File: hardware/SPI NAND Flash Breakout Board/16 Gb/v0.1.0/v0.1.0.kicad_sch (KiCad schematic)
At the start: 5 parts, among them J1 Conn_01x09_Pin, U1 AS5F18G04SND-10LIN, U2 TXB0108PW, U3 AS5F18G04SND-10LIN, U4 AP2127K-1.8

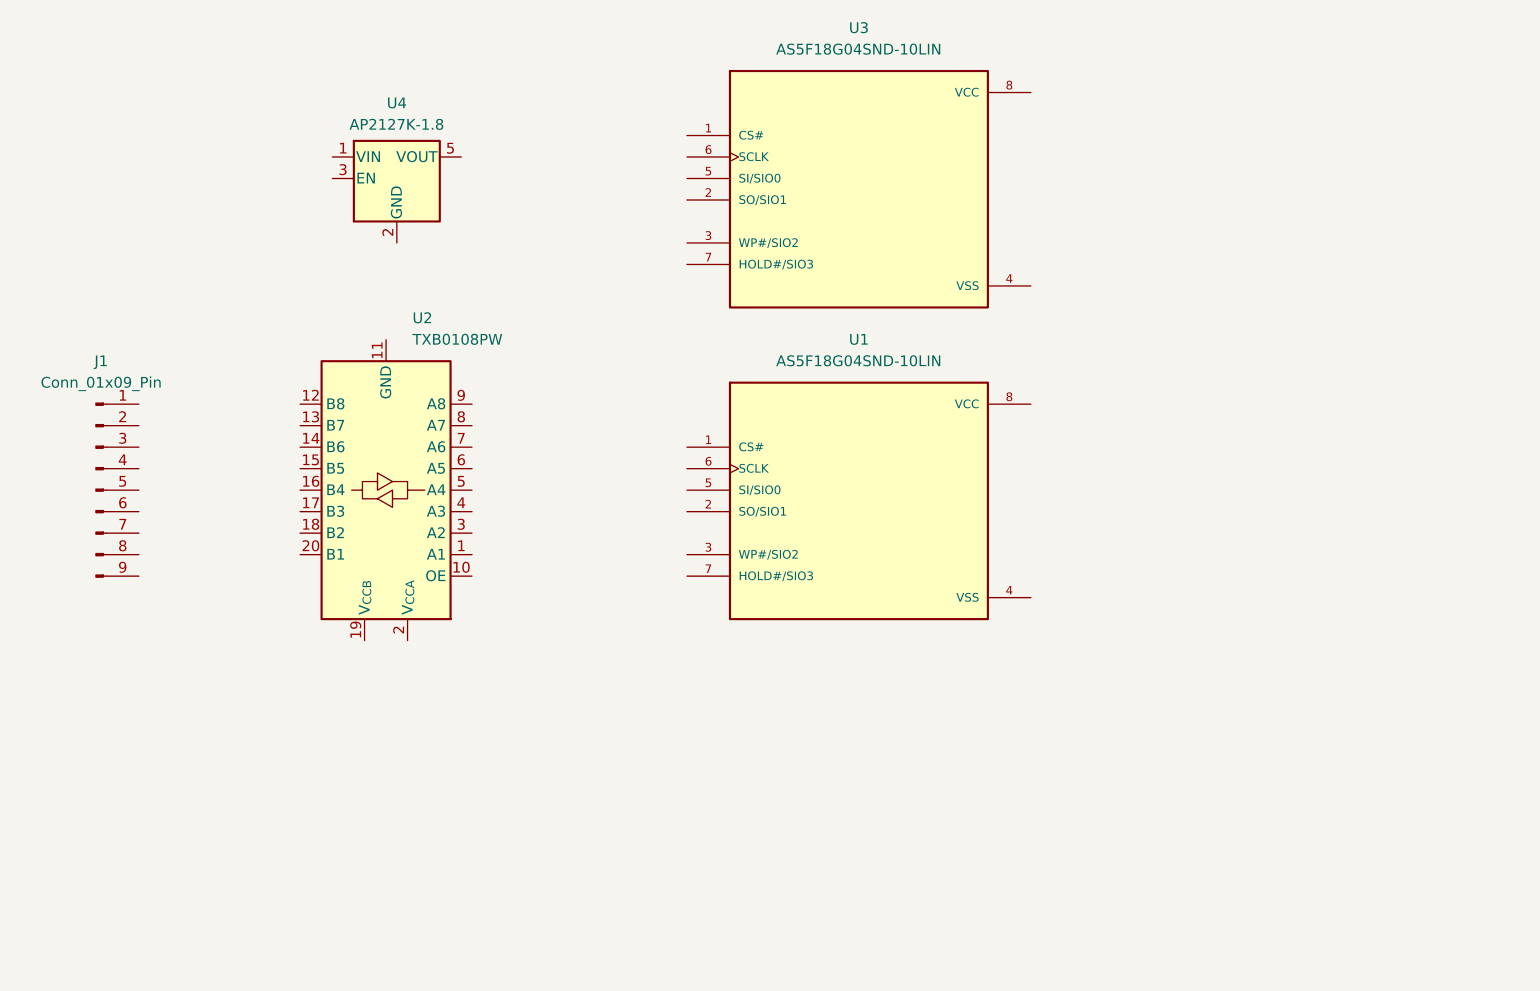
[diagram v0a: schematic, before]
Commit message: 16 Gb Design
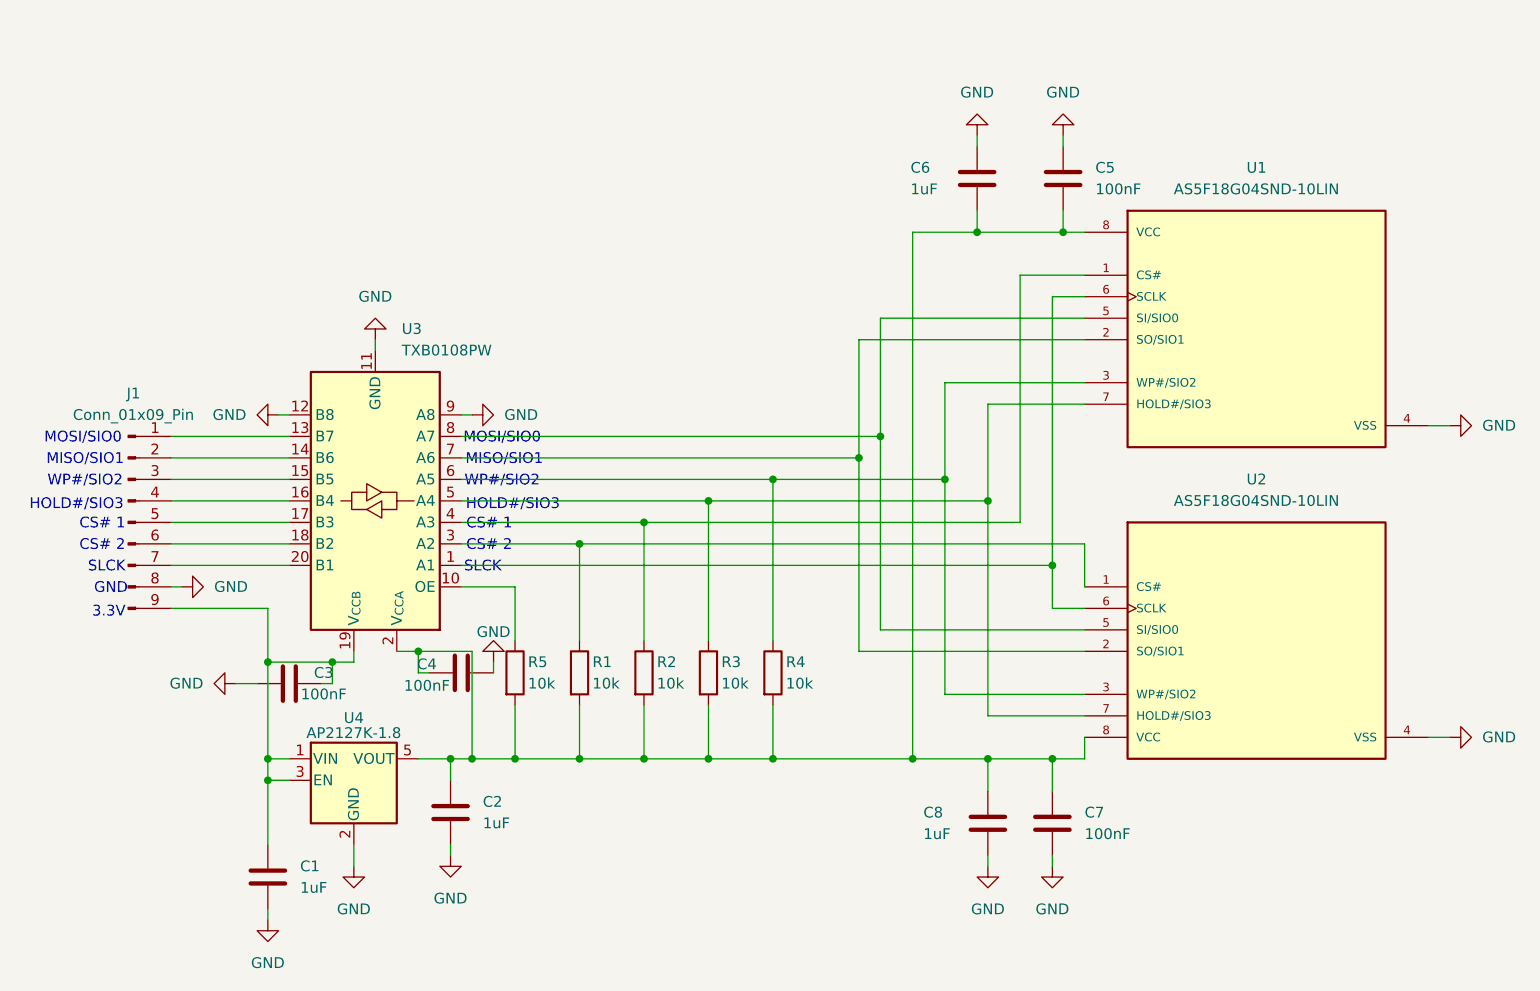
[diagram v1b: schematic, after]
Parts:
- added C1, C2, C6, C8: 1uF, Capacitor_SMD:C_0805_2012Metric, symbol Device:C
- added C3, C4, C5, C7: 100nF, Capacitor_SMD:C_0805_2012Metric, symbol Device:C
- added R1, R2, R3, R4, R5: 10k, Resistor_SMD:R_0805_2012Metric, symbol Device:R
- J1: footprint (none) -> Connector_PinSocket_2.54mm:PinSocket_1x09_P2.54mm_Vertical
- U1: renamed from U3; footprint AS5F18G04SND-10LIN:SON127P600X800X80-8N -> Breakout:SON127P600X800X80-8N
- U2: renamed from U1; footprint AS5F18G04SND-10LIN:SON127P600X800X80-8N -> Breakout:SON127P600X800X80-8N
- renumbered U2 to U3
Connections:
- net at U2.1 (CS#): now also U3.3 (A2), R1.1
- net at U2.2 (SO/SIO1): now also U1.2 (SO/SIO1), U3.7 (A6)
- net at U2.3 (WP#/SIO2): now also U1.3 (WP#/SIO2), U3.6 (A5), R4.1
- net GND: now reaches U2.4 (VSS)
- net GND: now also J1.8 (Pin_8), U1.4 (VSS), U3.11 (GND), U3.12 (B8), U3.9 (A8), U4.2 (GND), C1.2, C2.2, C3.1, C4.1, C5.1, C6.1, C7.2, C8.2
- net at U2.5 (SI/SIO0): now also U1.5 (SI/SIO0), U3.8 (A7)
- net at U2.6 (SCLK): now also U1.6 (SCLK), U3.1 (A1)
- net at U2.7 (HOLD#/SIO3): now also U1.7 (HOLD#/SIO3), U3.5 (A4), R3.1
- net at U2.8 (VCC): now also U1.8 (VCC), U3.2 (V_{CCA}), U4.5 (VOUT), C2.1, C4.2, C5.2, C6.2, C7.1, C8.1, R1.2, R2.2, R3.2, R4.2, R5.2
- net at J1.1 (Pin_1): now also U3.13 (B7)
- net at J1.2 (Pin_2): now also U3.14 (B6)
- net at J1.3 (Pin_3): now also U3.15 (B5)
- net at J1.4 (Pin_4): now also U3.16 (B4)
- net at J1.5 (Pin_5): now also U3.17 (B3)
- net at J1.6 (Pin_6): now also U3.18 (B2)
- net at J1.7 (Pin_7): now also U3.20 (B1)
- net at J1.9 (Pin_9): now also U3.19 (V_{CCB}), U4.1 (VIN), U4.3 (EN), C1.1, C3.2
- net at U3.10 (OE): now also R5.1
- net at U3.4 (A3): now also U1.1 (CS#), R2.1
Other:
- note added: "3.3V"
- note added: "CS# 1"
- note added: "CS# 2"
- note added: "GND"
- note added: "HOLD#/SIO3"
- note added: "MISO/SIO1"
- note added: "MOSI/SIO0"
- note added: "SLCK"
- note added: "WP#/SIO2"
- moved on the sheet: J1, U1, U2, U3, U4
